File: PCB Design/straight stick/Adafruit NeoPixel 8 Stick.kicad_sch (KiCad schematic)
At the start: 22 parts, among them CN1 1X4SMT, CN2 1X4SMT

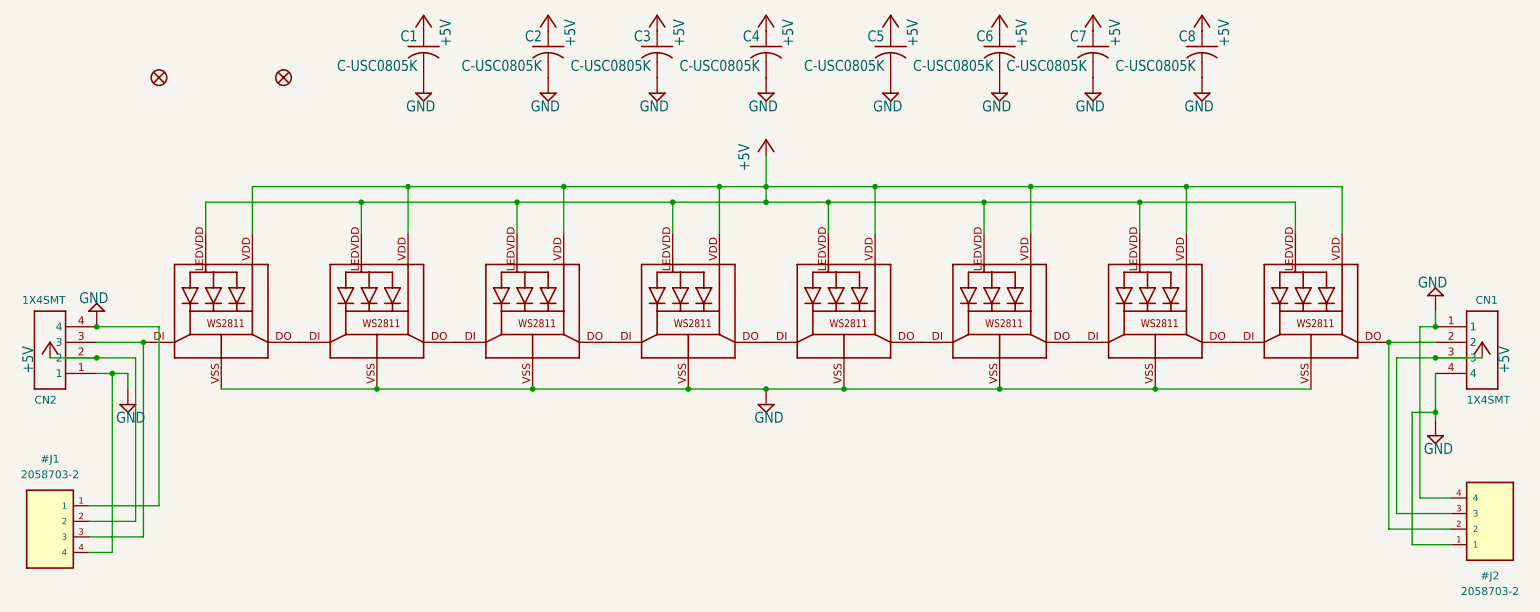
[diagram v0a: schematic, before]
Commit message: 4 pin fix
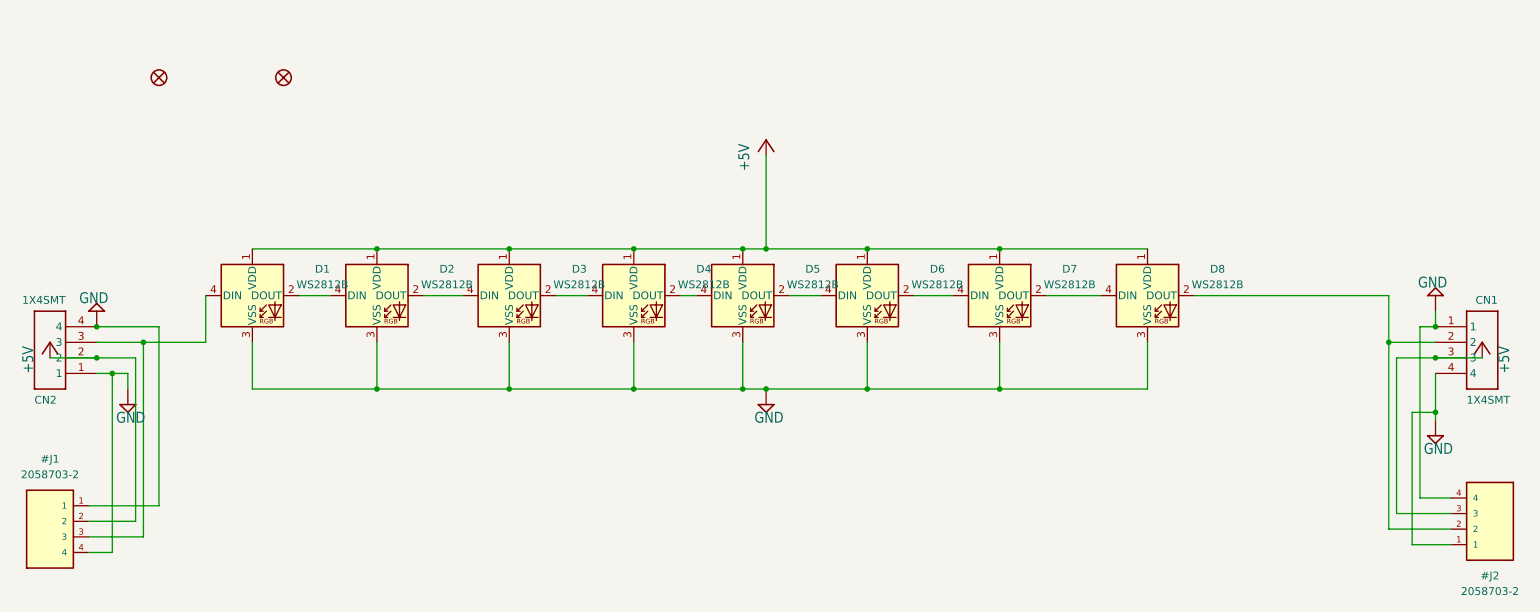
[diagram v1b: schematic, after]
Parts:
- removed C1, C2, C3, C4, C5, C6, C7, C8: C-USC0805K, Adafruit NeoPixel 8 Stick:C0805K, symbol Adafruit NeoPixel 8 Stick-eagle-import:C-USC0805K
- removed LED1, LED2, LED3, LED4, LED5, LED6, LED7, LED8: >VALUE, Adafruit NeoPixel 8 Stick:WS28115050, symbol Adafruit NeoPixel 8 Stick-eagle-import:WS28115050
- added D1, D2, D3, D4, D5, D6, D7, D8: WS2812B, LED_SMD:LED_WS2812B_PLCC4_5.0x5.0mm_P3.2mm, symbol LED:WS2812B
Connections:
- net +5V: now also D1.1 (VDD), D2.1 (VDD), D3.1 (VDD), D4.1 (VDD), D5.1 (VDD), D6.1 (VDD), D7.1 (VDD), D8.1 (VDD)
- net GND: now also D1.3 (VSS), D2.3 (VSS), D3.3 (VSS), D4.3 (VSS), D5.3 (VSS), D6.3 (VSS), D7.3 (VSS), D8.3 (VSS)
- net at #J1.3, CN2.3: now also D1.4 (DIN)
- net at #J2.2, CN1.2: now also D8.2 (DOUT)
- new net: D2.2 (DOUT), D3.4 (DIN)
- new net: D1.2 (DOUT), D2.4 (DIN)
- new net: D3.2 (DOUT), D4.4 (DIN)
- new net: D7.2 (DOUT), D8.4 (DIN)
- new net: D6.2 (DOUT), D7.4 (DIN)
- new net: D5.2 (DOUT), D6.4 (DIN)
- new net: D4.2 (DOUT), D5.4 (DIN)

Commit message: 6 pin
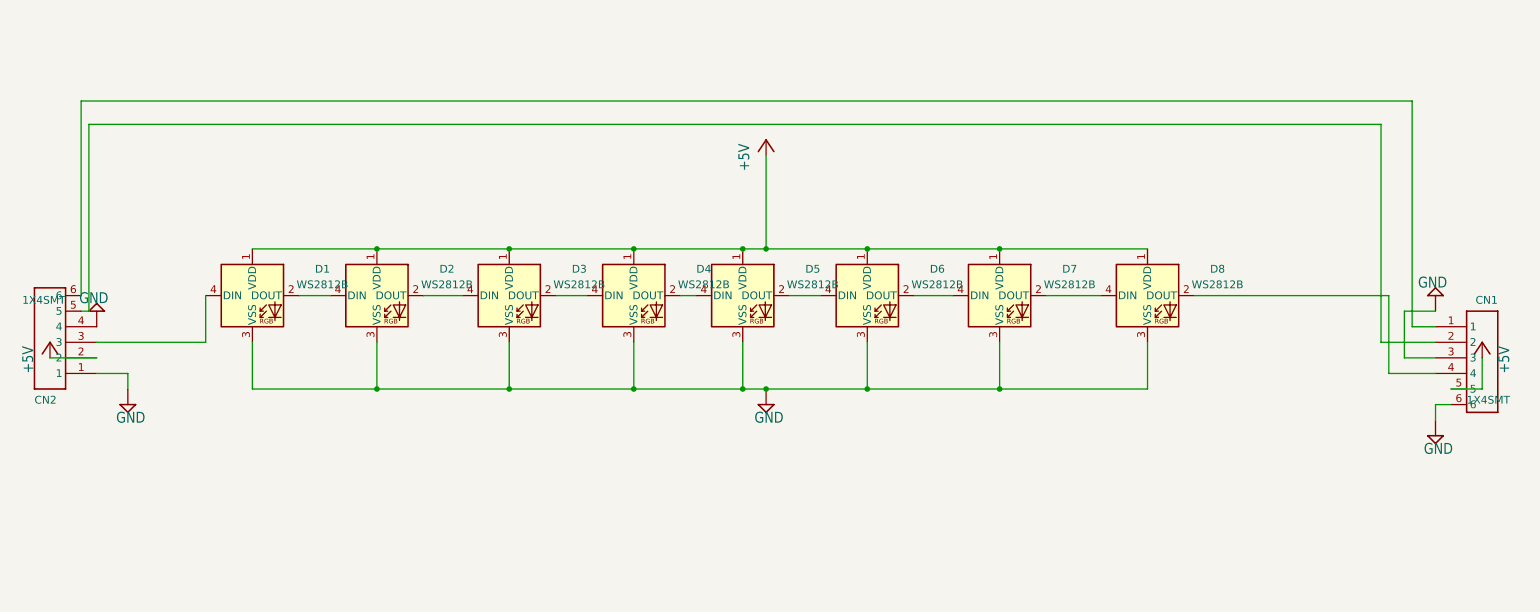
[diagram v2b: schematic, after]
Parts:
- removed #J1, #J2: 2058703-2, TE_2058703-2, symbol 2058703-2:2058703-2
- removed FID1, FID3: FIDUCIAL"", Adafruit NeoPixel 8 Stick:FIDUCIAL_1MM, symbol Adafruit NeoPixel 8 Stick-eagle-import:FIDUCIAL{dblquote}{dblquote}
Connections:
- net +5V: now also CN1.5; no longer CN1.3
- net GND: now also CN1.3, CN1.6; no longer CN1.1, CN1.4
- net at CN1.2: now also CN2.5; no longer D8.2 (DOUT)
- new net: CN1.1, CN2.6
- new net: CN1.4, D8.2 (DOUT)
